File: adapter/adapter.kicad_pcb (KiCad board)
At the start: 2 copper layers, 93.5 x 50.9 mm, 30 parts, among them J1 DF3A-2P-2DSA, J10 Ribbon, J11 Ribbon, J12 Ribbon, J2 DF3A-2P-2DSA, J9 Ribbon, SW1 CAS-120TA, SW2 CAS-120TA, U1 nice_nano, U2 nice_nano

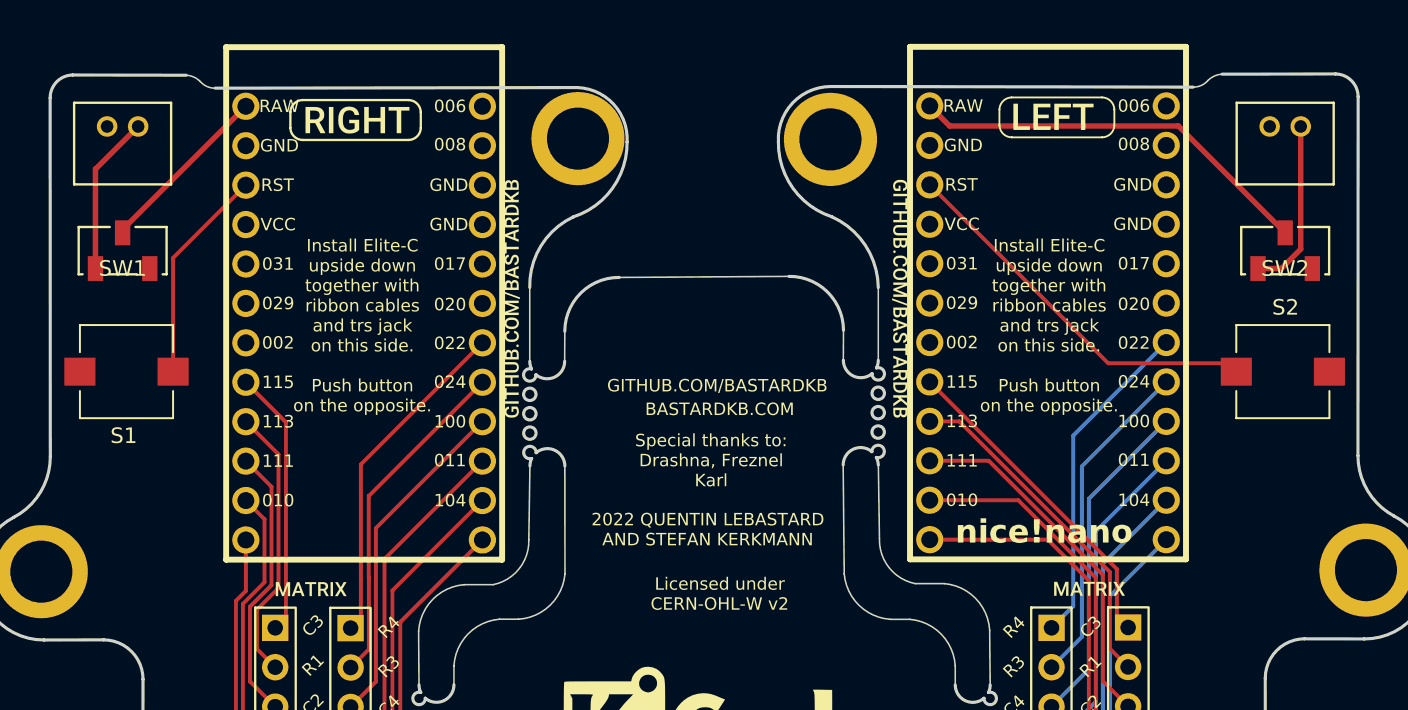
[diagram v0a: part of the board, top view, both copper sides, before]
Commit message: Cleanup the silk
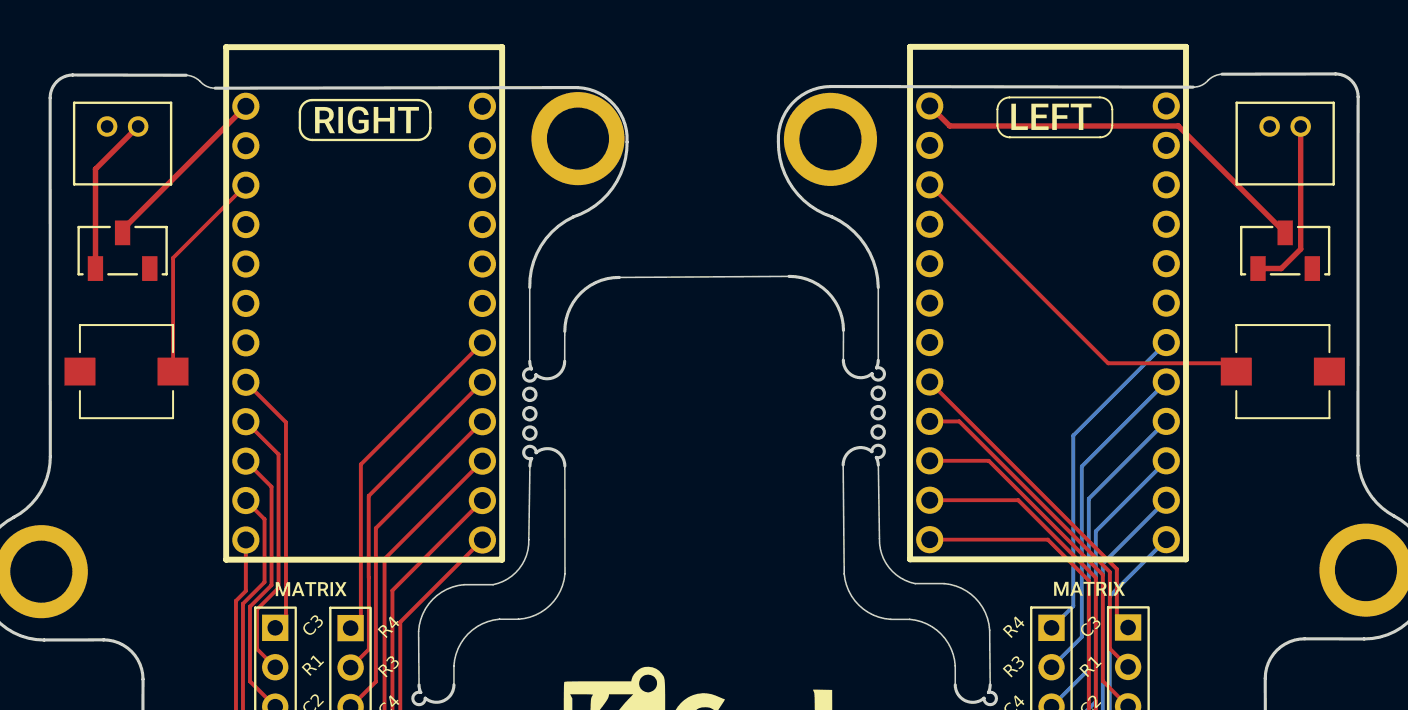
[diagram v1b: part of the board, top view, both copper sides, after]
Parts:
- removed kibuzzard-61F01A92 (x2): G***, kibuzzard-61F01A92
- removed kibuzzard-61F01C84 (x2): G***, kibuzzard-61F01C84
- moved kibuzzard-61F01B61 0.61 mm to (133.7, 70.1)
- moved kibuzzard-61F01B61 0.61 mm to (133.6, 70.1)
- moved kibuzzard-6208EFFE 0.13 mm to (177.8, 69.9)
- moved kibuzzard-6208EFFE 0.13 mm to (177.8, 70.1)
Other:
- board text removed: "Install Elite-C upside down together with ribbon cables and trs jack on this side. Push button on the opposite."
